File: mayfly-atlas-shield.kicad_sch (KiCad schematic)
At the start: 36 parts, among them J1 Conn_Coaxial, J2 Conn_Coaxial, J3 Conn_Coaxial, J4 Conn_Coaxial, J5 Conn_02x10_Counter_Clockwise, J6 Conn_02x10_Counter_Clockwise, U1 ISO1540, U2 CRE1S0505SC, U3 ISO1540, U4 CRE1S0505SC, U5 ISO1540, U6 CRE1S0505SC

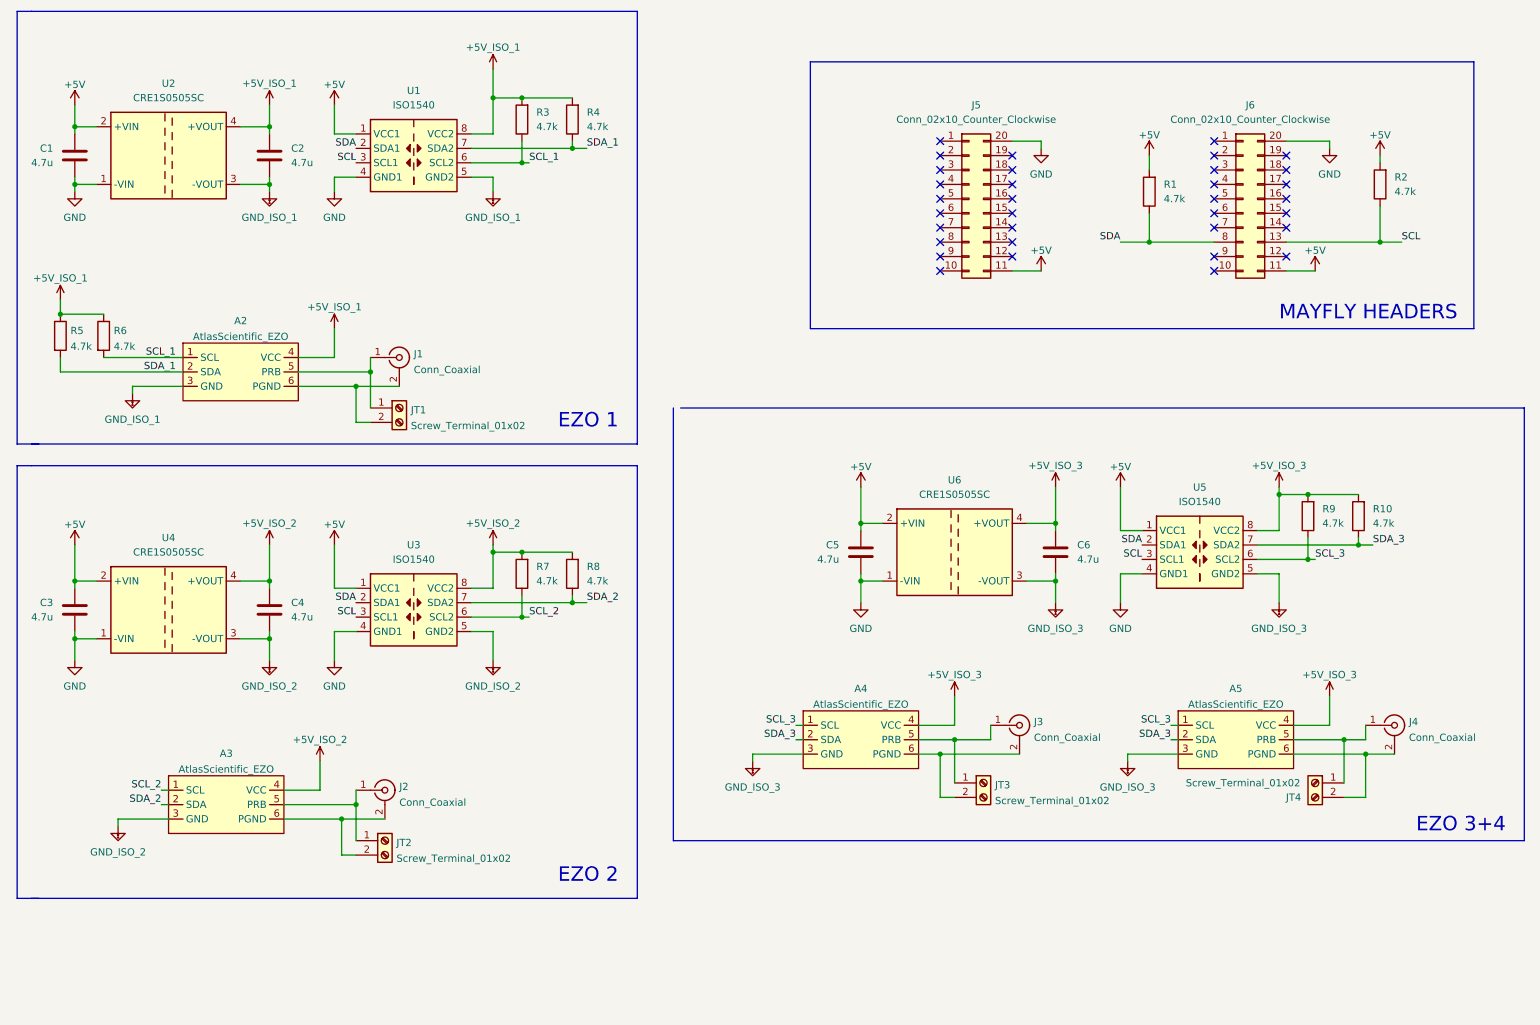
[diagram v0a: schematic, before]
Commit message: Revert "schematic finished"
This reverts commit 0515e0858473c3025873806ec2f0323e48e731ae.
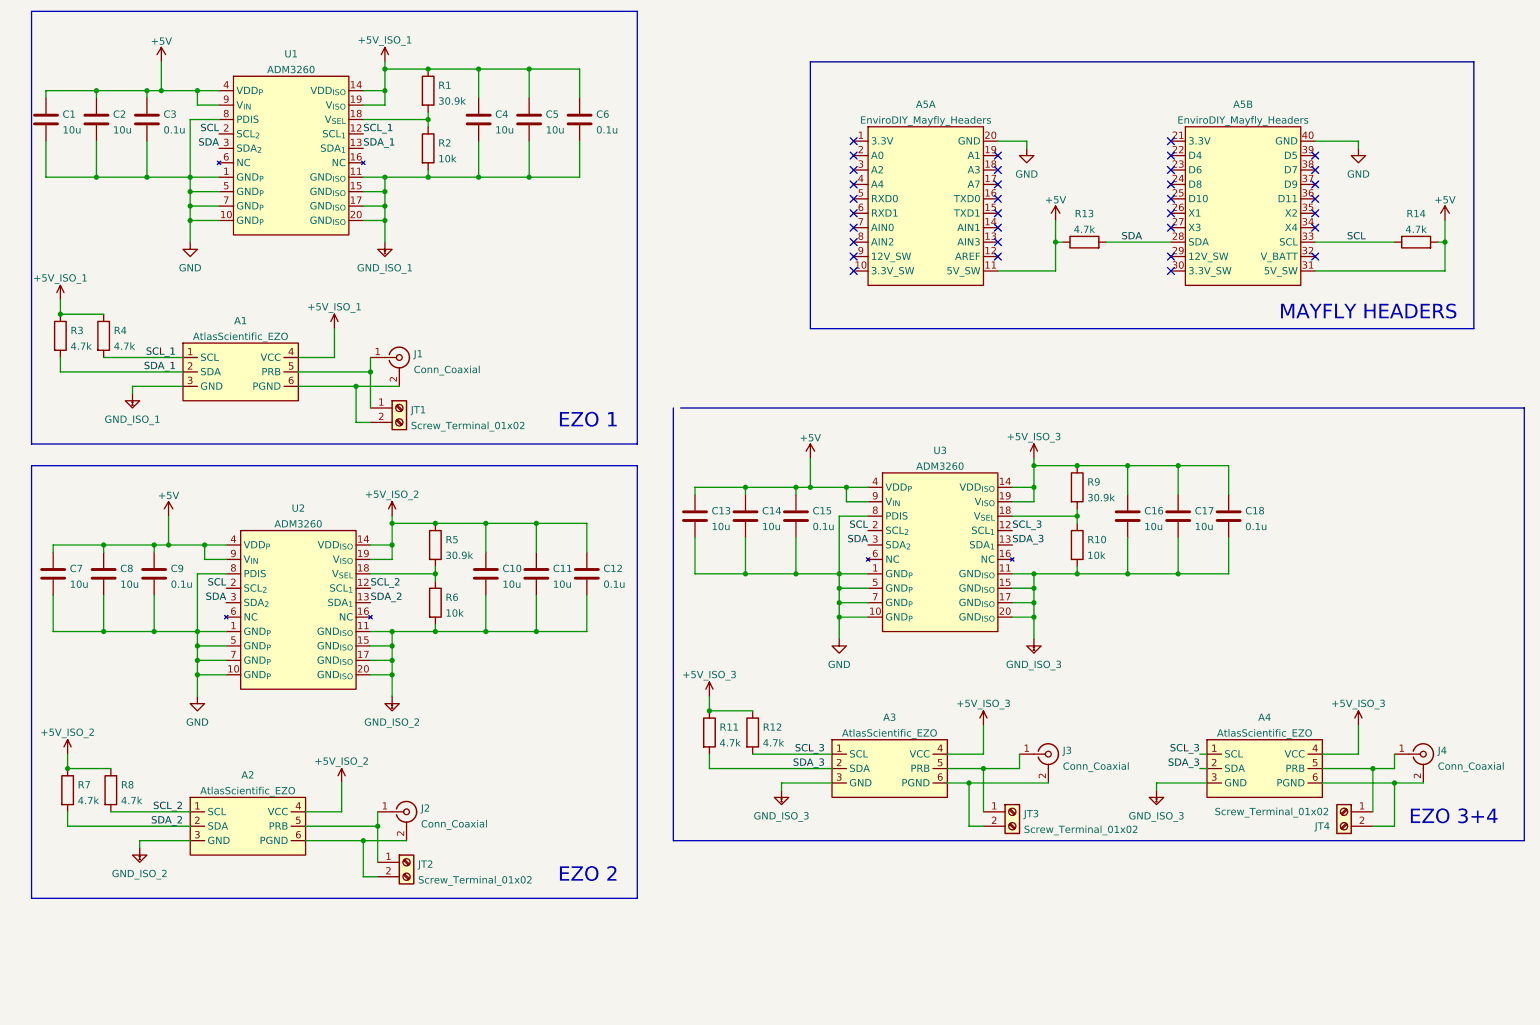
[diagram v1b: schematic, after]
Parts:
- removed J5, J6: Conn_02x10_Counter_Clockwise, toolbox-mayfly:Mayfly_v1_Headers, symbol Connector_Generic:Conn_02x10_Counter_Clockwise
- removed R3, R4: 4.7k, Resistor_SMD:R_0805_2012Metric, symbol Device:R
- removed U1, U3, U5: ISO1540, Package_SO:SOIC-8_3.9x4.9mm_P1.27mm, symbol Isolator:ISO1540
- removed U2, U4, U6: CRE1S0505SC, Converter_DCDC:Converter_DCDC_Murata_CRE1xxxxxxSC_THT, symbol Regulator_Switching:CRE1S0505SC
- added A5: EnviroDIY_Mayfly_Headers, symbol toolbox-assy:EnviroDIY_Mayfly_Headers
- added C10, C11, C13, C14, C16, C17, C7, C8: 10u, symbol Device:C
- added C12, C15, C18, C9: 0.1u, symbol Device:C
- added R1, R5: 30.9k, symbol Device:R
- added R11, R12: 4.7k, symbol Device:R
- added R2, R6: 10k, symbol Device:R
- added U1, U2, U3: ADM3260, symbol toolbox-ic:ADM3260
- A1: renamed from A2; footprint toolbox-mayfly:AtlasScientific_EZO -> (none)
- A2: renamed from A3; footprint toolbox-mayfly:AtlasScientific_EZO -> (none)
- A3: renamed from A4; footprint toolbox-mayfly:AtlasScientific_EZO -> (none)
- A4: renamed from A5; footprint toolbox-mayfly:AtlasScientific_EZO -> (none)
- C1, C2, C4, C5: value 4.7u -> 10u; footprint Capacitor_SMD:C_0805_2012Metric -> (none)
- C3, C6: value 4.7u -> 0.1u; footprint Capacitor_SMD:C_0805_2012Metric -> (none)
- J1, J2, J3, J4: footprint Connector_Coaxial:SMA_Amphenol_132134-16_Vertical -> (none)
- JT1, JT2, JT3, JT4: footprint TerminalBlock_Phoenix:TerminalBlock_Phoenix_PT-1,5-2-5.0-H_1x02_P5.00mm_Horizontal -> (none)
- R10: value 4.7k -> 10k; footprint Resistor_SMD:R_0805_2012Metric -> (none)
- R13: renamed from R2; footprint Resistor_SMD:R_0805_2012Metric -> (none)
- R14: renamed from R1; footprint Resistor_SMD:R_0805_2012Metric -> (none)
- R3: renamed from R5; footprint Resistor_SMD:R_0805_2012Metric -> (none)
- R4: renamed from R6; footprint Resistor_SMD:R_0805_2012Metric -> (none)
- R7, R8: footprint Resistor_SMD:R_0805_2012Metric -> (none)
- R9: value 4.7k -> 30.9k; footprint Resistor_SMD:R_0805_2012Metric -> (none)
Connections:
- net +5V: now also C1.1, C2.1, C3.1, R13.1, A5.11 (5V_SW), A5.31 (5V_SW), C13.1, C14.1, C15.1, C7.1, C8.1, C9.1, U1.4 (VDD_{P}), U1.9 (V_{IN}), U2.4 (VDD_{P}), U2.9 (V_{IN}), U3.4 (VDD_{P}), U3.9 (V_{IN}); no longer C1.2, C3.2, C5.2, R13.2
- net +5V_ISO_1: now also C4.1, C5.1, C6.1, R1.1, U1.14 (VDD_{ISO}), U1.19 (V_{ISO}); no longer C2.1
- net +5V_ISO_2: now also R7.1, R8.1, C10.1, C11.1, C12.1, R5.1, U2.14 (VDD_{ISO}), U2.19 (V_{ISO}); no longer C4.1, R7.2, R8.2
- net +5V_ISO_3: now also R9.1, C16.1, C17.1, C18.1, R11.1, R12.1, U3.14 (VDD_{ISO}), U3.19 (V_{ISO}); no longer C6.1, R10.2, R9.2
- net GND: now also C1.2, C2.2, C3.2, A5.20 (GND), A5.40 (GND), C13.2, C14.2, C15.2, C7.2, C8.2, C9.2, U1.1 (GND_{P}), U1.10 (GND_{P}), U1.5 (GND_{P}), U1.7 (GND_{P}), U1.8 (PDIS), U2.1 (GND_{P}), U2.10 (GND_{P}), U2.5 (GND_{P}), U2.7 (GND_{P}), U2.8 (PDIS), U3.1 (GND_{P}), U3.10 (GND_{P}), U3.5 (GND_{P}), U3.7 (GND_{P}), U3.8 (PDIS); no longer C1.1, C3.1, C5.1
- net GND_ISO_1: now also C4.2, C5.2, C6.2, R2.2, U1.11 (GND_{ISO}), U1.15 (GND_{ISO}), U1.17 (GND_{ISO}), U1.20 (GND_{ISO}); no longer C2.2
- net GND_ISO_2: now also C10.2, C11.2, C12.2, R6.2, U2.11 (GND_{ISO}), U2.15 (GND_{ISO}), U2.17 (GND_{ISO}), U2.20 (GND_{ISO}); no longer C4.2
- net GND_ISO_3: now also R10.2, C16.2, C17.2, C18.2, U3.11 (GND_{ISO}), U3.15 (GND_{ISO}), U3.17 (GND_{ISO}), U3.20 (GND_{ISO}); no longer C6.2
- net SCL: now also R14.1, A5.33 (SCL), U1.2 (SCL_{2}), U2.2 (SCL_{2}), U3.2 (SCL_{2}); no longer R13.1
- net SCL_1: now also U1.12 (SCL_{1})
- net SCL_2: now also R8.2, U2.12 (SCL_{1}); no longer R7.1
- net SCL_3: now also R12.2, U3.12 (SCL_{1}); no longer R9.1
- net SDA: now also R13.2, A5.28 (SDA), U1.3 (SDA_{2}), U2.3 (SDA_{2}), U3.3 (SDA_{2}); no longer R14.1
- net SDA_1: now also U1.13 (SDA_{1})
- net SDA_2: now also R7.2, U2.13 (SDA_{1}); no longer R8.1
- net SDA_3: now also R11.2, U3.13 (SDA_{1}); no longer R10.1
- new net: R1.2, R2.1, U1.18 (V_{SEL})
- new net: R10.1, R9.2, U3.18 (V_{SEL})
- new net: R5.2, R6.1, U2.18 (V_{SEL})
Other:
- moved on the sheet: A2, A3, A4, J2, J3, J4, JT2, JT3, JT4, R13, R14

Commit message: schematic finished
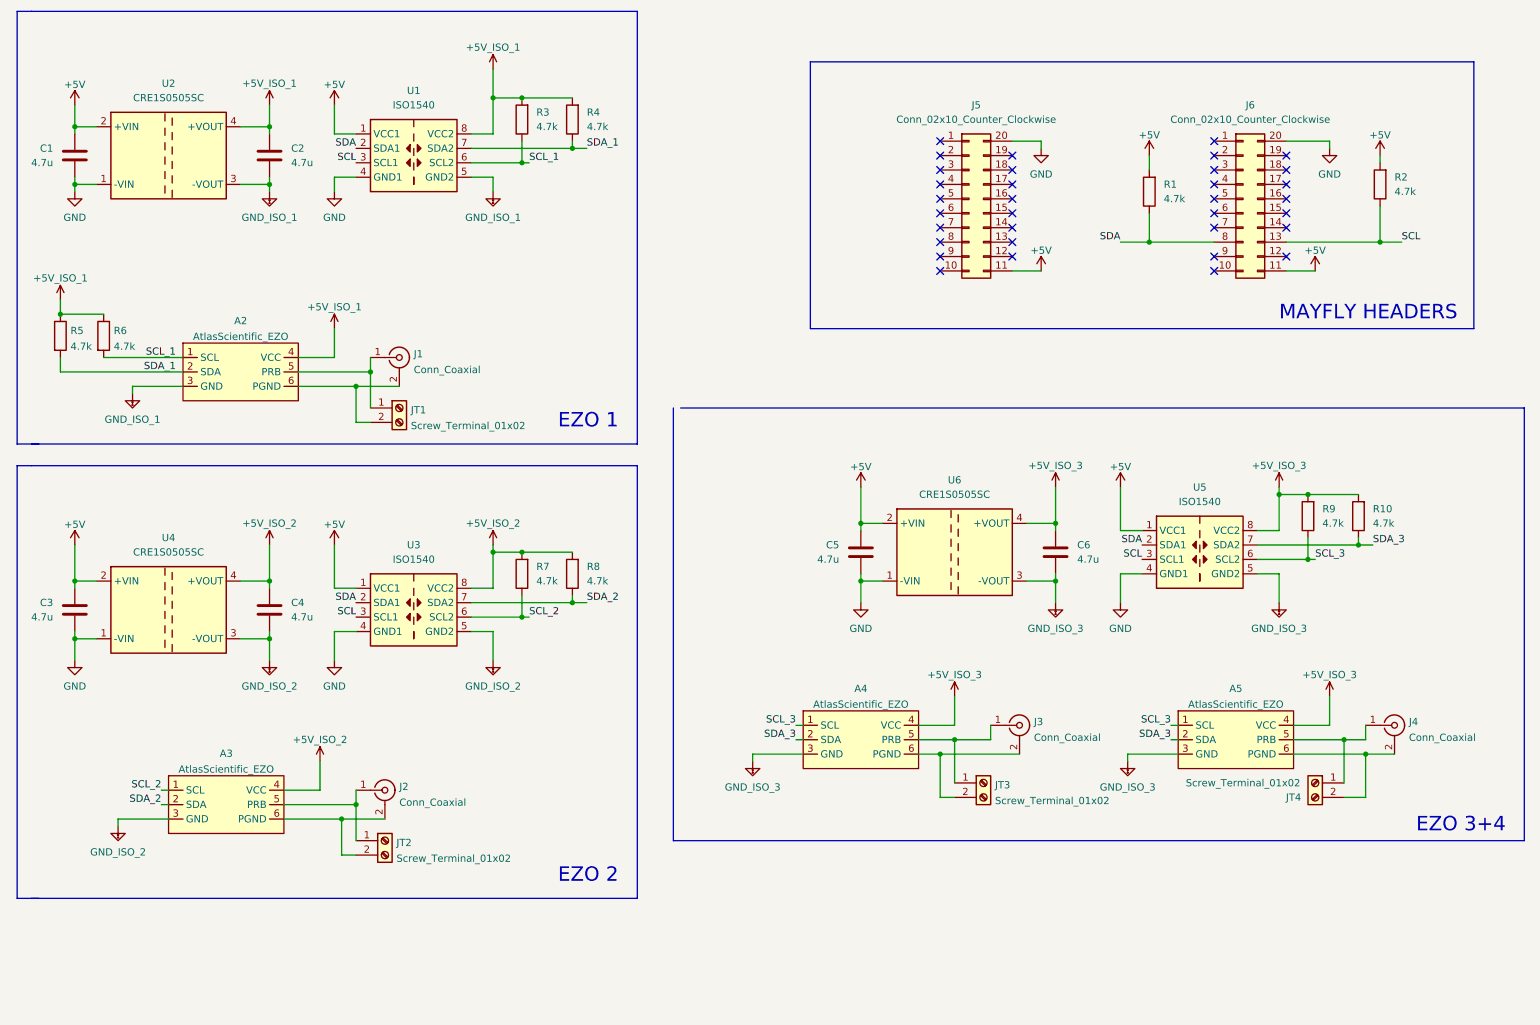
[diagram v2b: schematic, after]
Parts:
- removed A5: EnviroDIY_Mayfly_Headers, symbol toolbox-assy:EnviroDIY_Mayfly_Headers
- removed C10, C11, C13, C14, C16, C17, C7, C8: 10u, symbol Device:C
- removed C12, C15, C18, C9: 0.1u, symbol Device:C
- removed R1, R5: 30.9k, symbol Device:R
- removed R11, R12: 4.7k, symbol Device:R
- removed R2, R6: 10k, symbol Device:R
- removed U1, U2, U3: ADM3260, symbol toolbox-ic:ADM3260
- added J5, J6: Conn_02x10_Counter_Clockwise, toolbox-mayfly:Mayfly_v1_Headers, symbol Connector_Generic:Conn_02x10_Counter_Clockwise
- added R3, R4: 4.7k, Resistor_SMD:R_0805_2012Metric, symbol Device:R
- added U1, U3, U5: ISO1540, Package_SO:SOIC-8_3.9x4.9mm_P1.27mm, symbol Isolator:ISO1540
- added U2, U4, U6: CRE1S0505SC, Converter_DCDC:Converter_DCDC_Murata_CRE1xxxxxxSC_THT, symbol Regulator_Switching:CRE1S0505SC
- A2: renamed from A1; footprint (none) -> toolbox-mayfly:AtlasScientific_EZO
- A3: renamed from A2; footprint (none) -> toolbox-mayfly:AtlasScientific_EZO
- A4: renamed from A3; footprint (none) -> toolbox-mayfly:AtlasScientific_EZO
- A5: renamed from A4; footprint (none) -> toolbox-mayfly:AtlasScientific_EZO
- C1, C2, C4, C5: value 10u -> 4.7u; footprint (none) -> Capacitor_SMD:C_0805_2012Metric
- C3, C6: value 0.1u -> 4.7u; footprint (none) -> Capacitor_SMD:C_0805_2012Metric
- J1, J2, J3, J4: footprint (none) -> Connector_Coaxial:SMA_Amphenol_132134-16_Vertical
- JT1, JT2, JT3, JT4: footprint (none) -> TerminalBlock_Phoenix:TerminalBlock_Phoenix_PT-1,5-2-5.0-H_1x02_P5.00mm_Horizontal
- R1: renamed from R14; footprint (none) -> Resistor_SMD:R_0805_2012Metric
- R10: value 10k -> 4.7k; footprint (none) -> Resistor_SMD:R_0805_2012Metric
- R2: renamed from R13; footprint (none) -> Resistor_SMD:R_0805_2012Metric
- R5: renamed from R3; footprint (none) -> Resistor_SMD:R_0805_2012Metric
- R6: renamed from R4; footprint (none) -> Resistor_SMD:R_0805_2012Metric
- R7, R8: footprint (none) -> Resistor_SMD:R_0805_2012Metric
- R9: value 30.9k -> 4.7k; footprint (none) -> Resistor_SMD:R_0805_2012Metric
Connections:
- net +5V: now also C1.2, C3.2, C5.2, R2.2, J5.11 (Pin_11), J6.11 (Pin_11), U1.1 (VCC1), U2.2 (+VIN), U3.1 (VCC1), U4.2 (+VIN), U5.1 (VCC1), U6.2 (+VIN); no longer C1.1, C2.1, C3.1, R2.1
- net +5V_ISO_1: now also C2.1, R3.2, R4.2, U1.8 (VCC2), U2.4 (+VOUT); no longer C4.1, C5.1, C6.1
- net +5V_ISO_2: now also C4.1, R7.2, R8.2, U3.8 (VCC2), U4.4 (+VOUT); no longer R7.1, R8.1
- net +5V_ISO_3: now also C6.1, R10.2, R9.2, U5.8 (VCC2), U6.4 (+VOUT); no longer R9.1
- net GND: now also C1.1, C3.1, C5.1, J5.20 (Pin_20), J6.20 (Pin_20), U1.4 (GND1), U2.1 (-VIN), U3.4 (GND1), U4.1 (-VIN), U5.4 (GND1), U6.1 (-VIN); no longer C1.2, C2.2, C3.2
- net GND_ISO_1: now also C2.2, U1.5 (GND2), U2.3 (-VOUT); no longer C4.2, C5.2, C6.2
- net GND_ISO_2: now also C4.2, U3.5 (GND2), U4.3 (-VOUT)
- net GND_ISO_3: now also C6.2, U5.5 (GND2), U6.3 (-VOUT); no longer R10.2
- net SCL: now also R2.1, J6.13 (Pin_13), U1.3 (SCL1), U3.3 (SCL1), U5.3 (SCL1); no longer R1.1
- net SCL_1: now also R3.1, U1.6 (SCL2)
- net SCL_2: now also R7.1, U3.6 (SCL2); no longer R8.2
- net SCL_3: now also R9.1, U5.6 (SCL2)
- net SDA: now also R1.1, J6.8 (Pin_8), U1.2 (SDA1), U3.2 (SDA1), U5.2 (SDA1); no longer R2.2
- net SDA_1: now also R4.1, U1.7 (SDA2)
- net SDA_2: now also R8.1, U3.7 (SDA2); no longer R7.2
- net SDA_3: now also R10.1, U5.7 (SDA2)
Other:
- moved on the sheet: A3, A4, A5, J2, J3, J4, JT2, JT3, JT4, R1, R2

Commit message: pcb layout
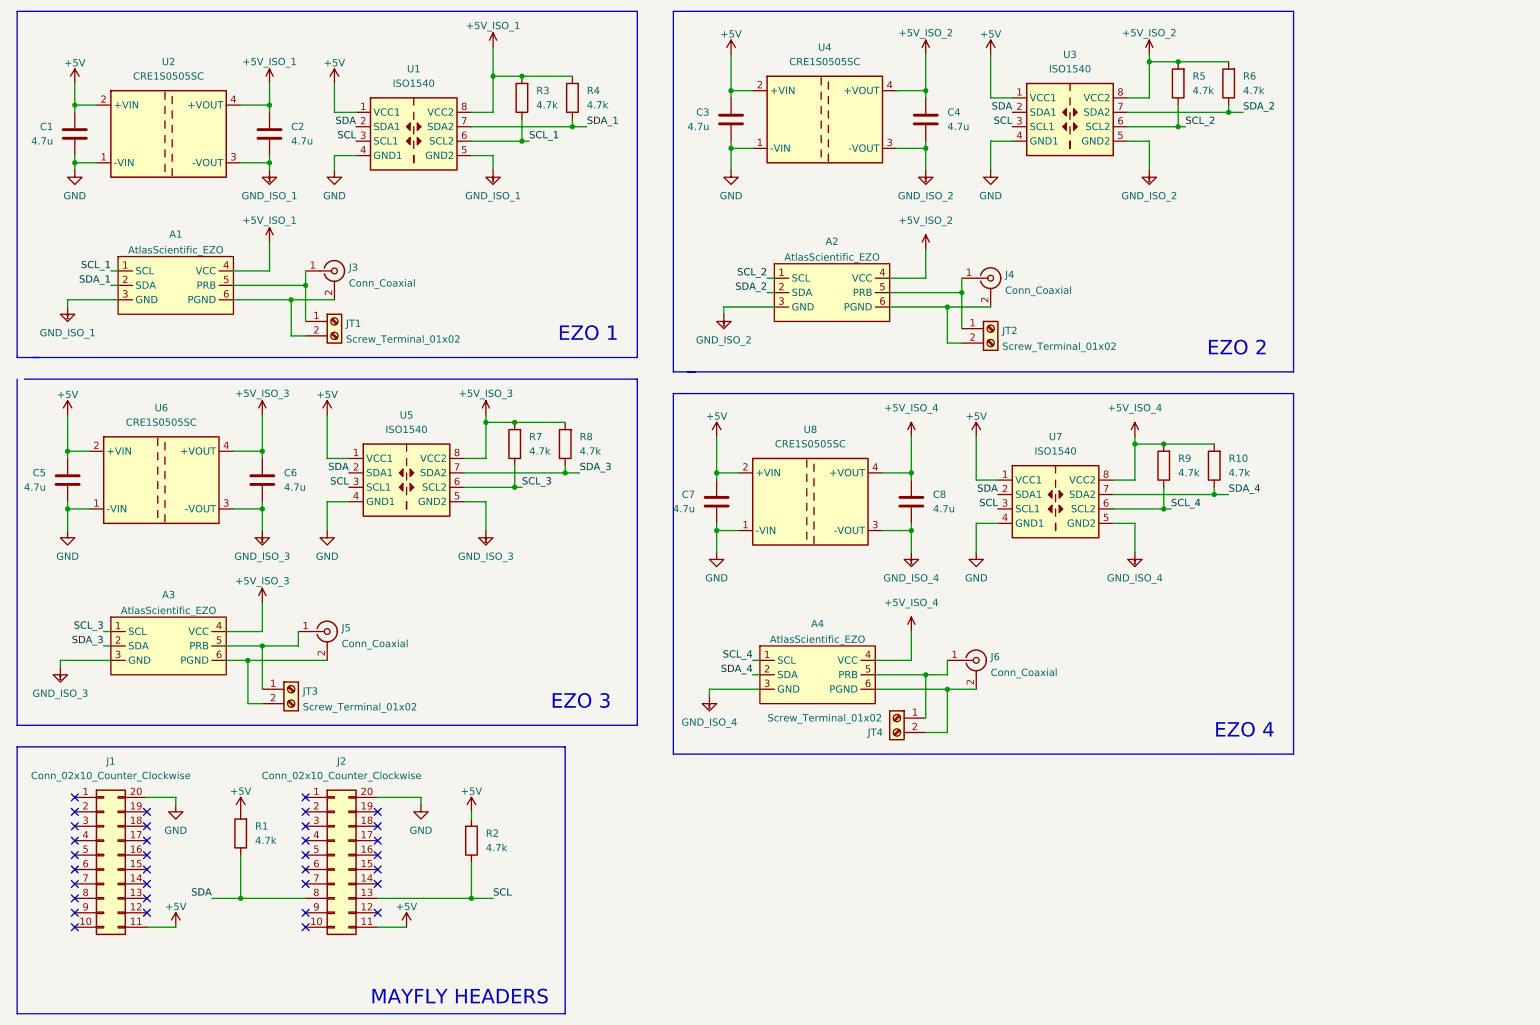
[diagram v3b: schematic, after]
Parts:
- removed R5, R6: 4.7k, Resistor_SMD:R_0805_2012Metric, symbol Device:R
- added C7, C8: 4.7u, Capacitor_SMD:C_0805_2012Metric, symbol Device:C
- added R10, R9: 4.7k, Resistor_SMD:R_0805_2012Metric, symbol Device:R
- added U7: ISO1540, Package_SO:SOIC-8_3.9x4.9mm_P1.27mm, symbol Isolator:ISO1540
- added U8: CRE1S0505SC, Converter_DCDC:Converter_DCDC_Murata_CRE1xxxxxxSC_THT, symbol Regulator_Switching:CRE1S0505SC
- renumbered A2 to A1, A3 to A2, A4 to A3, A5 to A4, J5 to J1, J6 to J2, J1 to J3, J2 to J4, J3 to J5, J4 to J6, R7 to R5, R8 to R6, R9 to R7, R10 to R8
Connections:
- net +5V: now also C7.2, U7.1 (VCC1), U8.2 (+VIN)
- net +5V_ISO_3: no longer A4.4 (VCC)
- net GND: now also C7.1, U7.4 (GND1), U8.1 (-VIN)
- net GND_ISO_3: no longer A4.3 (GND)
- net SCL: now also U7.3 (SCL1)
- net SCL_3: no longer A4.1 (SCL)
- net SDA: now also U7.2 (SDA1)
- net SDA_3: no longer A4.2 (SDA)
- new net +5V_ISO_4: A4.4 (VCC), C8.1, R10.2, R9.2, U7.8 (VCC2), U8.4 (+VOUT)
- new net GND_ISO_4: A4.3 (GND), C8.2, U7.5 (GND2), U8.3 (-VOUT)
- new net SCL_4: A4.1 (SCL), R9.1, U7.6 (SCL2)
- new net SDA_4: A4.2 (SDA), R10.1, U7.7 (SDA2)
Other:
- note added: "EZO 3"
- note added: "EZO 4"
- note removed: "EZO 3+4"
- moved on the sheet: A1, A2, A3, A4, C1, C2, C3, C4, C5, C6, J1, J2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
